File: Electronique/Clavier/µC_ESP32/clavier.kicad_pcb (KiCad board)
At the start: 2 copper layers, 65 x 46 mm, 46 parts, among them J4 Conn_02x13_Odd_Even, Q1 2N7002, Q2 SI2365EDS, SW74 SW_Push_SPDT, U1 USBLC6-2P6, U2 MCP73871-2CC, U4 ESP32-S3-WROOM-1

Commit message: global update
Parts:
- removed H1, H2, H3, H4: MountingHole_Pad, MountingHole:MountingHole_3.2mm_M3_DIN965_Pad
- moved R19 191.5 mm to (121.3, 79.6)
- moved BOOT1 191.5 mm to (119.7, 71.5)
- moved C1 191.5 mm to (89.5, 76.5)
- moved C12 191.5 mm to (94.9, 68.7)
- moved C13 191.5 mm to (93.4, 68.7)
- moved C14 191.5 mm to (118.2, 83.0)
- moved C15 191.5 mm to (90.4, 73.9)
- moved C2 191.5 mm to (91.9, 68.7)
- moved C3 191.5 mm to (90.4, 68.7)
- moved J4 191.5 mm to (78.8, 72.4)
- moved PS1 191.5 mm to (87.3, 70.5)
- moved R20 191.5 mm to (118.3, 84.8)
- moved R21 191.5 mm to (92.2, 72.2)
- moved RST1 191.5 mm to (94.1, 77.6)
- moved U4 191.5 mm to (106.5, 73.6)
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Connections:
- U4 pad 34: unconnected-(U4-IO41-Pad34) -> L1
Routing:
- net L1: track 0.00 -> 58.1 mm, vias 0 -> 1
- net Vusb: track 57.9 -> 67.6 mm
- net Col11: track 68.7 -> 60.5 mm
- net GND: track 2.44 -> 7.02 mm, vias 11 -> 51
- net Net-(U2-VPCC): track 4.22 -> 8.23 mm
- net Vol_Down: track 23.7 -> 20.3 mm
- net Net-(J1-CC1): track 3.38 -> 6.69 mm
- net Net-(J1-CC2): track 3.77 -> 6.59 mm
- net Col10: track 38.2 -> 40.4 mm
- net PG: track 50.0 -> 48.8 mm
- net Valim: track 57.0 -> 56.0 mm
- net L4: track 52.7 -> 53.7 mm
- net Vbat+: track 21.4 -> 20.6 mm
- net Net-(U2-PROG3): track 4.35 -> 3.67 mm
- net Col12: track 40.1 -> 40.6 mm
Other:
- board size 65 x 46 mm -> 52 x 51.7 mm

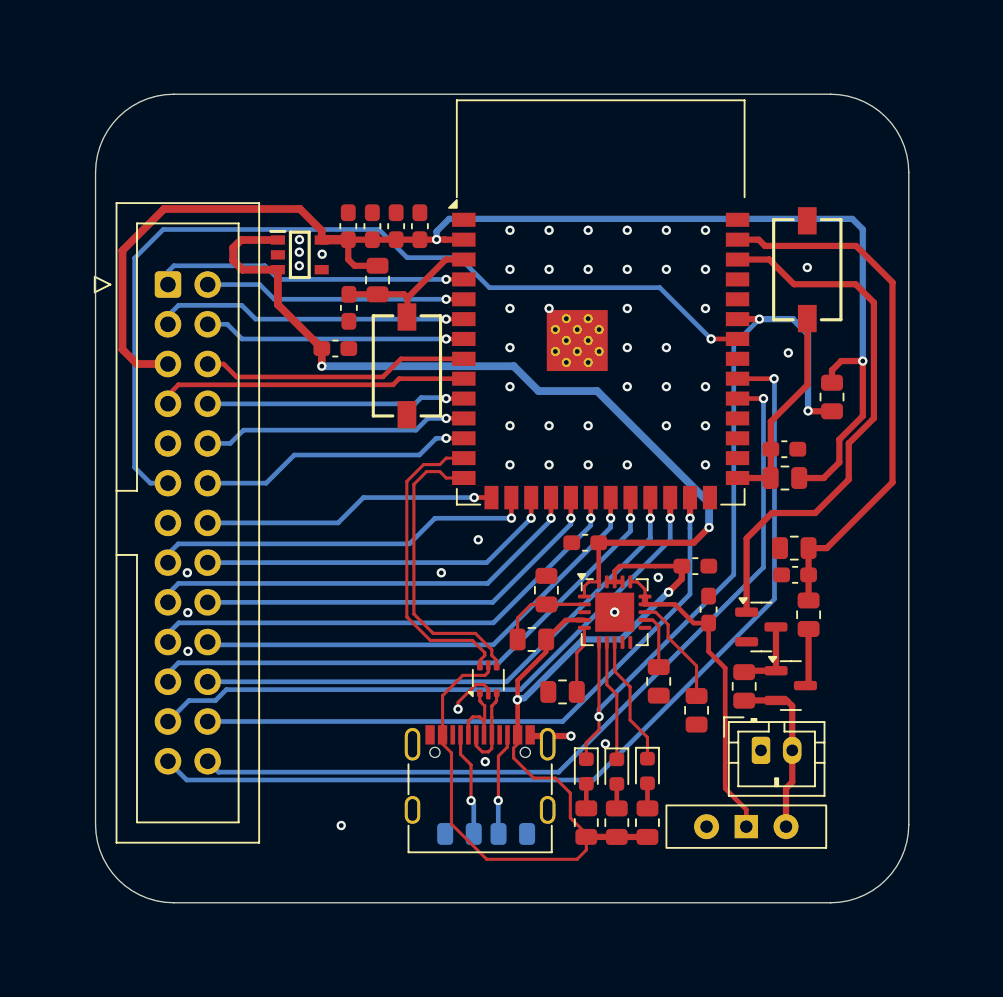
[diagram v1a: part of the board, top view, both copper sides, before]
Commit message: mm
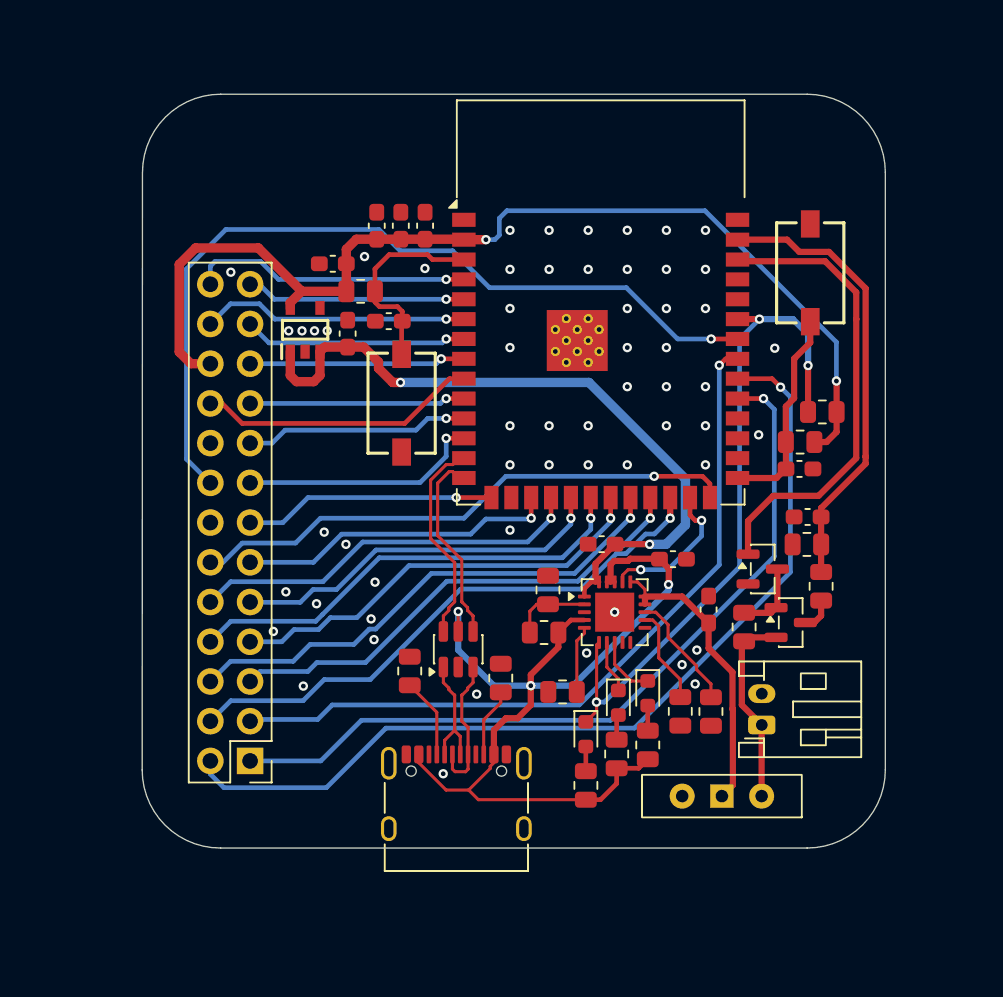
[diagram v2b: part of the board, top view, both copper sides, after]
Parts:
- removed C14: 100nF, Capacitor_SMD:C_0603_1608Metric_Pad1.08x0.95mm_HandSolder
- removed J1: ~, Connector_USB:USB_C_Receptacle_G-Switch_GT-USB-7010ASV
- removed R15, R16: 100k, Resistor_SMD:R_0805_2012Metric
- removed R17: 220k, Resistor_SMD:R_0805_2012Metric
- removed R19: 10K, Resistor_SMD:R_0805_2012Metric
- removed R20: 10k, Resistor_SMD:R_0805_2012Metric
- added C7: 100nF, Capacitor_SMD:C_0603_1608Metric_Pad1.08x0.95mm_HandSolder, F.Cu at (119.2, 84.2)
- added J2: Conn_02x13_Odd_Even, Connector_PinHeader_2.54mm:PinHeader_2x13_P2.54mm_Vertical, F.Cu at (84.1, 102.9)
- added R11: 100k, Resistor_SMD:R_0805_2012Metric, F.Cu at (115.7, 94.3)
- added R12: 27k, Resistor_SMD:R_0805_2012Metric, F.Cu at (120.6, 91.7)
- added R13: 68k, Resistor_SMD:R_0805_2012Metric, F.Cu at (119.7, 89.1)
- added R8: 10K, Resistor_SMD:R_0805_2012Metric, F.Cu at (120.7, 80.6)
- added R9: 10k, Resistor_SMD:R_0805_2012Metric, F.Cu at (119.2, 82.5)
- J3: renamed from J2; footprint Connector_JST:JST_PH_B2B-PH-K_1x02_P2.00mm_Vertical -> Connector_JST:JST_PH_S2B-PH-K_1x02_P2.00mm_Horizontal
- J4: value Conn_02x13_Odd_Even -> USB_C_Receptacle_USB2.0_14P; footprint Connector_IDC:IDC-Header_2x13_P2.54mm_Vertical -> Connector_USB:USB_C_Receptacle_XKB_U262-16XN-4BVC11
- R1, R2: moved to F.Cu
- Rprog1: renamed from R12; value 2k -> 3k3
- Rprog3: renamed from R11; value 20k -> 3k3
- U1: footprint Package_TO_SOT_SMD:SOT-666 -> Package_TO_SOT_SMD:SOT-23-6
- moved J4 38.4 mm to (97.3, 106.2)
- moved R1 10.9 mm to (94.3, 97.2), turned to 90 degrees
- moved R2 10.00 mm to (100.1, 97.6), turned to 90 degrees
- moved C5 6.07 mm to (89.4, 71.1), turned to 0 degrees
- moved R5 4.97 mm to (109.5, 101.9)
- moved STAT1 4.97 mm to (109.5, 98.6)
- moved PS1 4.80 mm to (87.6, 75.3), turned to 90 degrees
- moved STAT2 4.40 mm to (107.6, 99.2)
- moved R6 4.39 mm to (107.5, 102.5)
- moved Q2 4.03 mm to (118.7, 94.0)
- moved C11 3.79 mm to (119.7, 87.3)
- moved Q1 3.70 mm to (116.9, 90.6)
- moved C2 3.37 mm to (95.3, 68.7)
- moved C3 3.36 mm to (93.7, 68.7)
- moved U1 2.75 mm to (97.4, 95.8)
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- renumbered C9 to C10, C12 to C5, C13 to C6, C15 to C8, C8 to C9, R21 to R10, R4 to R3, R5 to R4, R6 to R5, R7 to R6, R9 to R7, R13 to Rtherm1, SW74 to SW1, U4 to U2, U2 to U3
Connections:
- net Valim renamed VCC
- net Vbat+ renamed +BATT
- C4 pad 1: Vusb -> VBUS
- J3 pad 1: GND -> Vbat_Mes
- J3 pad 2: Vbat_Mes -> GND
- R1 pad 1: Net-(J1-CC1) -> Net-(J4-CC1)
- R2 pad 1: Net-(J1-CC2) -> Net-(J4-CC2)
- R3 pad 1: Vusb -> VBUS
- R4 pad 1: Vusb -> VBUS
- R5 pad 1: Vusb -> VBUS
- R6 pad 1: Vusb -> VBUS
- U1 pad 5: Vusb -> VBUS
- U2 pad 16: L5 -> unconnected-(U2-IO46-Pad16)
- U2 pad 25: Col10 -> CE
- U2 pad 26: unconnected-(U4-IO45-Pad26) -> L5
- U2 pad 33: unconnected-(U4-IO40-Pad33) -> Col10
- U3 pad 17: Vusb -> CE
- U3 pad 18: Vusb -> VBUS
- U3 pad 19: Vusb -> VBUS
- U3 pad 4: Vusb -> VBUS
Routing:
- net Vusb: track 67.6 -> 0.00 mm, vias 2 -> 0
- net VBUS: track 0.00 -> 60.5 mm, vias 0 -> 3
- net +3.3V: track 86.9 -> 68.2 mm
- net VCC: track 56.0 -> 45.1 mm
- net L5: track 24.8 -> 35.3 mm
- net CE: track 0.00 -> 9.53 mm, vias 0 -> 2
- net Col10: track 40.4 -> 48.2 mm
- net GND: track 7.02 -> 0.00 mm, vias 51 -> 58
- net Net-(J1-CC1): track 6.69 -> 0.00 mm, vias 1 -> 0
- net Net-(J1-CC2): track 6.59 -> 0.00 mm, vias 1 -> 0
- net DP+: track 19.1 -> 12.6 mm
- net DP-: track 19.9 -> 13.3 mm
- net Check Batt: track 34.3 -> 28.8 mm
- net Net-(J4-CC1): track 0.00 -> 5.08 mm
- net Check Batt En: track 34.6 -> 29.8 mm
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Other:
- board size 52 x 51.7 mm -> 47.5 x 48.2 mm
- board text added: "BOOT"
- board text added: "RST"
